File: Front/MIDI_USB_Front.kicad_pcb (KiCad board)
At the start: 2 copper layers, 20 x 128.5 mm, 7 parts, among them J1 Jack_3.5mm, J2 Jack_3.5mm, J3 Jack_3.5mm, J4 Jack_3.5mm

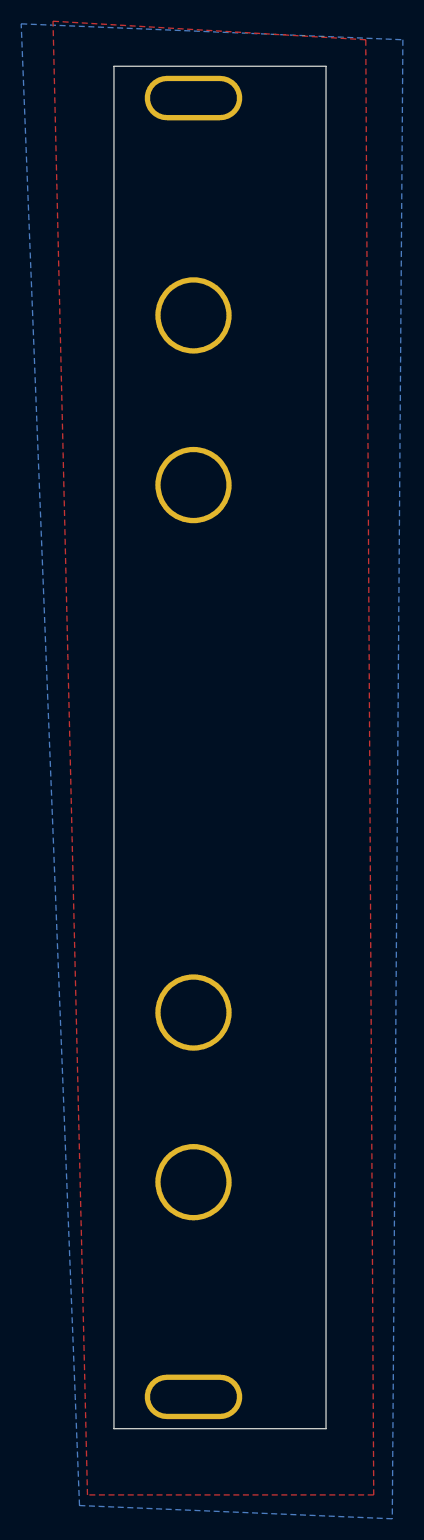
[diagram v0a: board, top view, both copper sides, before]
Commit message: Update front panel layout
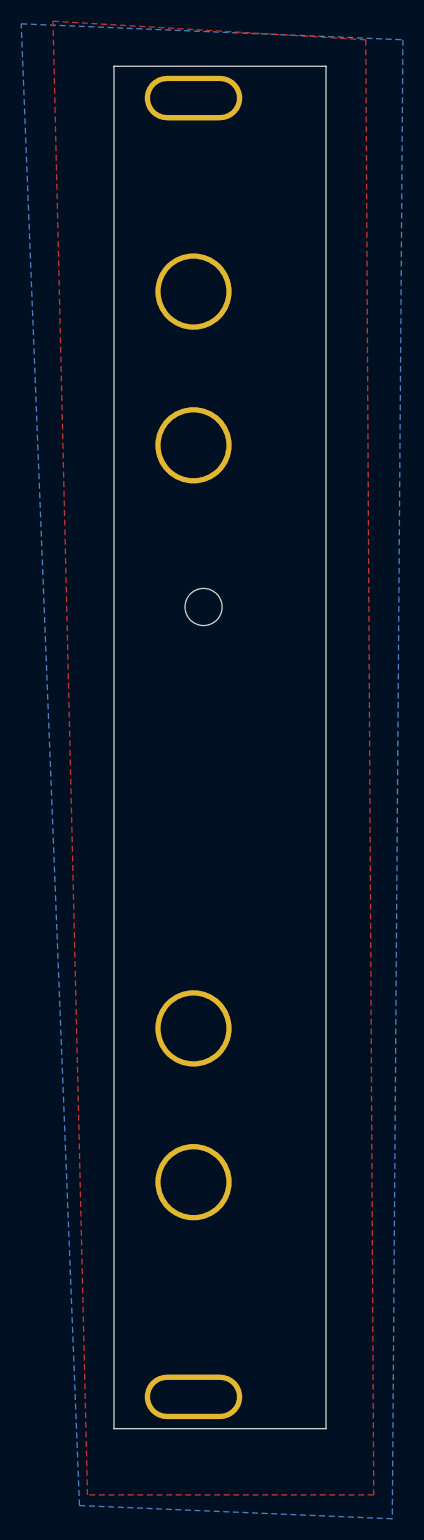
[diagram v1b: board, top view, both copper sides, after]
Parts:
- added H4: Tactile hole, Custom_FP:TactileHole, F.Cu at (108.5, 101.0)
- moved J1 3.75 mm to (107.5, 85.8)
- moved J3 2.25 mm to (107.5, 71.2)
- moved J2 1.50 mm to (107.5, 140.8)
- moved H1 0.30 mm to (110.6, 120.8)
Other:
- board text added: "L"
- board text added: "L(/R)"
- board text added: "R"

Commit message: Re-arrange USB components
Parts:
- added G***: LOGO, GuavTek_Logo:GuavTek_Logo_Mask, F.Cu at (110.0, 168.0)
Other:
- rule pad_to_mask_clearance: 0.05 -> 0

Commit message: Adjust 5V power protection
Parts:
- removed G***: LOGO, GuavTek_Logo:GuavTek_Logo_Mask
